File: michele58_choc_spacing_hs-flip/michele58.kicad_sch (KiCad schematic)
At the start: 103 parts, among them J1 OLED, J2 i2c, J3 i2c, J4 LED, U1 EliteC_Pro_Micro, U2 TRRS

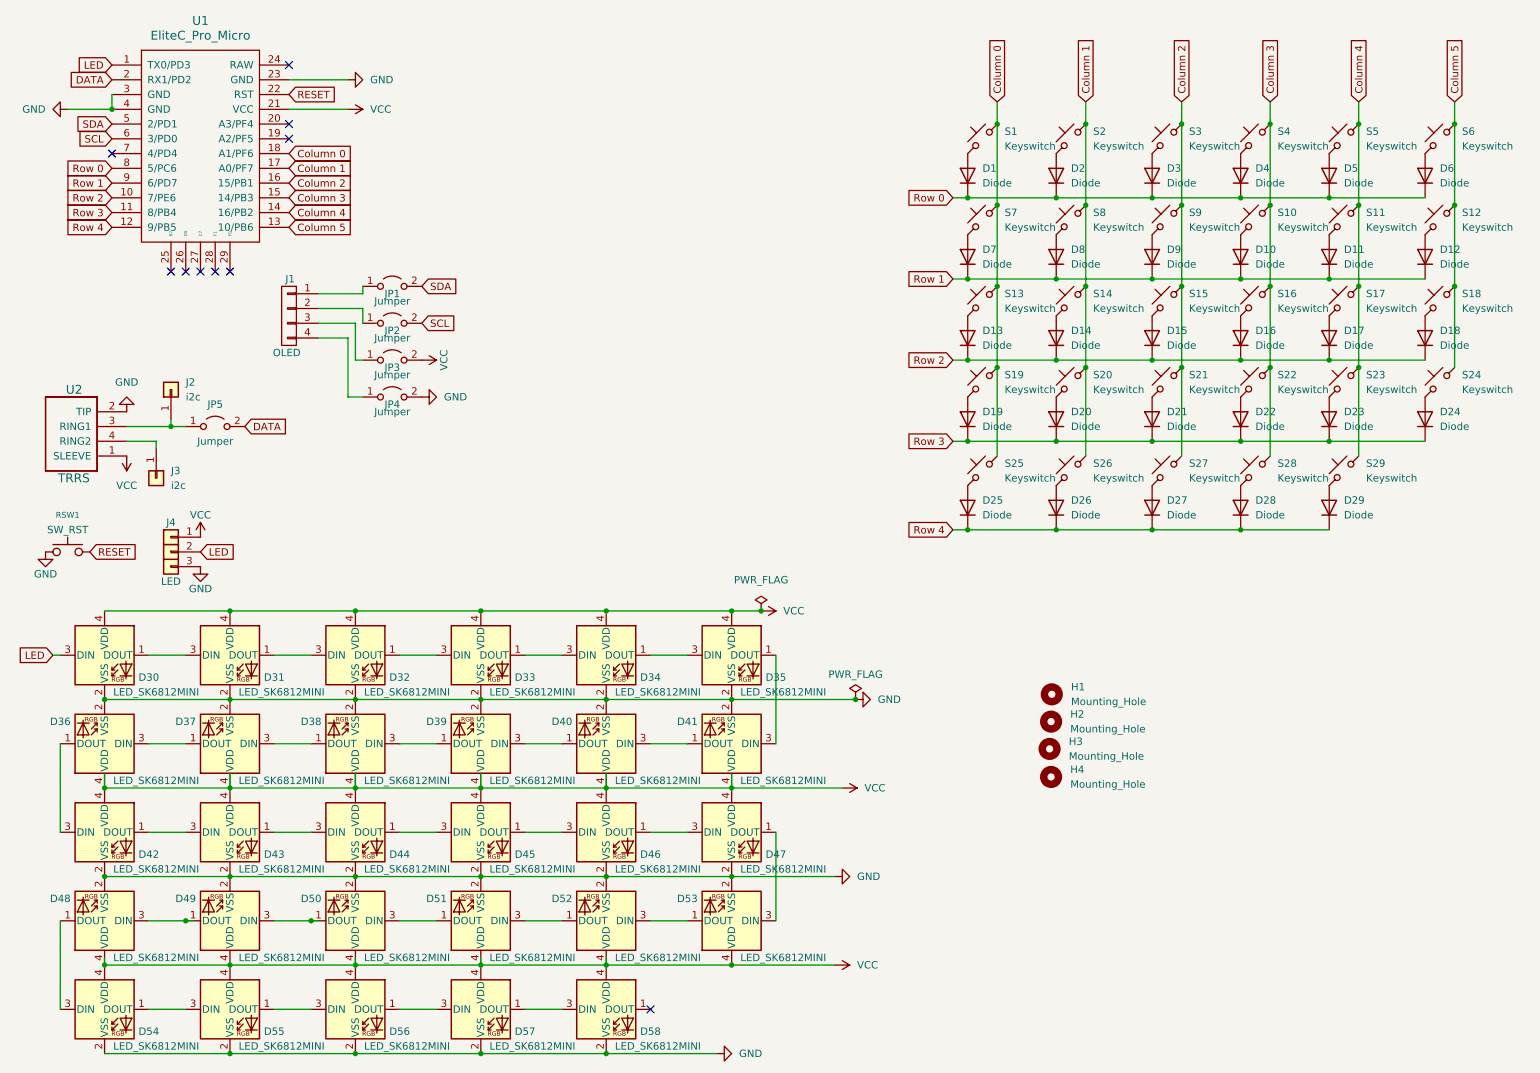
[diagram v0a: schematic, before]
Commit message: latest changes
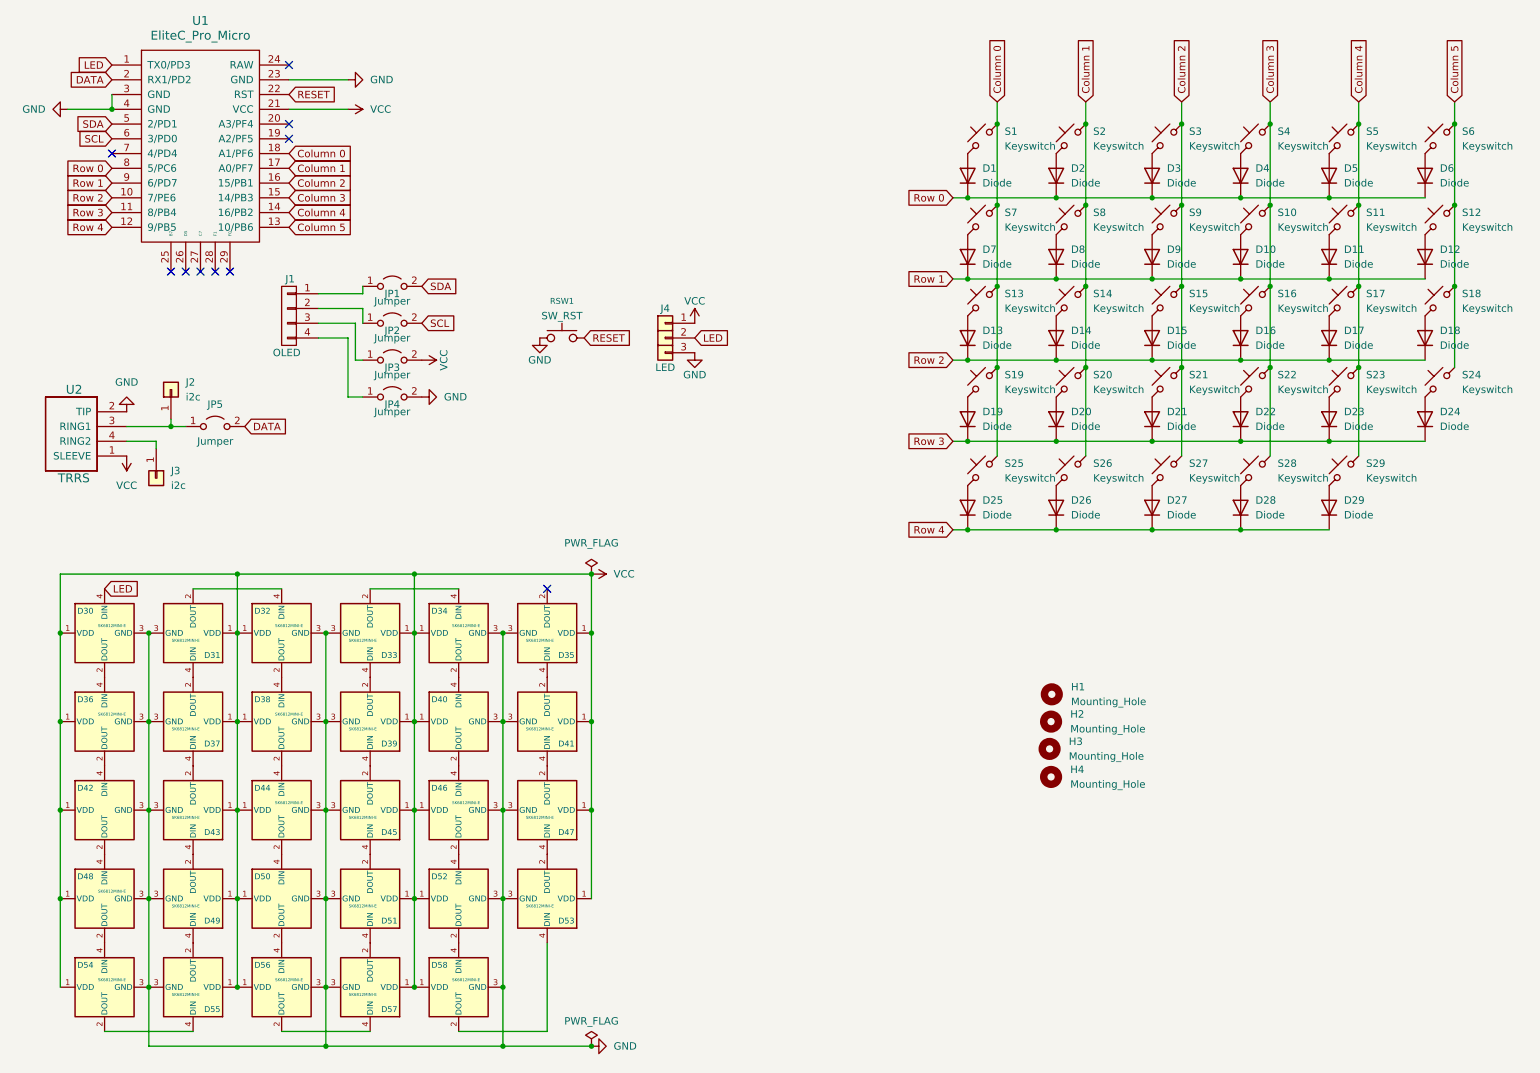
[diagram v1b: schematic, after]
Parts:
- D30: value LED_SK6812MINI -> SK6812MINI-E; symbol ScottoKeebs:LED_SK6812MINI -> SofleKeyboard1:LED_SK6812MINI-E-alt
- D31: renamed from D36; value LED_SK6812MINI -> SK6812MINI-E; symbol ScottoKeebs:LED_SK6812MINI -> SofleKeyboard1:LED_SK6812MINI-E-alt
- D32: renamed from D42; value LED_SK6812MINI -> SK6812MINI-E; symbol ScottoKeebs:LED_SK6812MINI -> SofleKeyboard1:LED_SK6812MINI-E-alt
- D33: renamed from D48; value LED_SK6812MINI -> SK6812MINI-E; symbol ScottoKeebs:LED_SK6812MINI -> SofleKeyboard1:LED_SK6812MINI-E-alt
- D34: renamed from D54; value LED_SK6812MINI -> SK6812MINI-E; symbol ScottoKeebs:LED_SK6812MINI -> SofleKeyboard1:LED_SK6812MINI-E-alt
- D35: renamed from D31; value LED_SK6812MINI -> SK6812MINI-E; symbol ScottoKeebs:LED_SK6812MINI -> SofleKeyboard1:LED_SK6812MINI-E-alt
- D36: renamed from D37; value LED_SK6812MINI -> SK6812MINI-E; symbol ScottoKeebs:LED_SK6812MINI -> SofleKeyboard1:LED_SK6812MINI-E-alt
- D37: renamed from D43; value LED_SK6812MINI -> SK6812MINI-E; symbol ScottoKeebs:LED_SK6812MINI -> SofleKeyboard1:LED_SK6812MINI-E-alt
- D38: renamed from D49; value LED_SK6812MINI -> SK6812MINI-E; symbol ScottoKeebs:LED_SK6812MINI -> SofleKeyboard1:LED_SK6812MINI-E-alt
- D39: renamed from D55; value LED_SK6812MINI -> SK6812MINI-E; symbol ScottoKeebs:LED_SK6812MINI -> SofleKeyboard1:LED_SK6812MINI-E-alt
- D40: renamed from D32; value LED_SK6812MINI -> SK6812MINI-E; symbol ScottoKeebs:LED_SK6812MINI -> SofleKeyboard1:LED_SK6812MINI-E-alt
- D41: renamed from D38; value LED_SK6812MINI -> SK6812MINI-E; symbol ScottoKeebs:LED_SK6812MINI -> SofleKeyboard1:LED_SK6812MINI-E-alt
- D42: renamed from D44; value LED_SK6812MINI -> SK6812MINI-E; symbol ScottoKeebs:LED_SK6812MINI -> SofleKeyboard1:LED_SK6812MINI-E-alt
- D43: renamed from D50; value LED_SK6812MINI -> SK6812MINI-E; symbol ScottoKeebs:LED_SK6812MINI -> SofleKeyboard1:LED_SK6812MINI-E-alt
- D44: renamed from D56; value LED_SK6812MINI -> SK6812MINI-E; symbol ScottoKeebs:LED_SK6812MINI -> SofleKeyboard1:LED_SK6812MINI-E-alt
- D45: renamed from D33; value LED_SK6812MINI -> SK6812MINI-E; symbol ScottoKeebs:LED_SK6812MINI -> SofleKeyboard1:LED_SK6812MINI-E-alt
- D46: renamed from D39; value LED_SK6812MINI -> SK6812MINI-E; symbol ScottoKeebs:LED_SK6812MINI -> SofleKeyboard1:LED_SK6812MINI-E-alt
- D47: renamed from D45; value LED_SK6812MINI -> SK6812MINI-E; symbol ScottoKeebs:LED_SK6812MINI -> SofleKeyboard1:LED_SK6812MINI-E-alt
- D48: renamed from D51; value LED_SK6812MINI -> SK6812MINI-E; symbol ScottoKeebs:LED_SK6812MINI -> SofleKeyboard1:LED_SK6812MINI-E-alt
- D49: renamed from D57; value LED_SK6812MINI -> SK6812MINI-E; symbol ScottoKeebs:LED_SK6812MINI -> SofleKeyboard1:LED_SK6812MINI-E-alt
- D50: renamed from D34; value LED_SK6812MINI -> SK6812MINI-E; symbol ScottoKeebs:LED_SK6812MINI -> SofleKeyboard1:LED_SK6812MINI-E-alt
- D51: renamed from D40; value LED_SK6812MINI -> SK6812MINI-E; symbol ScottoKeebs:LED_SK6812MINI -> SofleKeyboard1:LED_SK6812MINI-E-alt
- D52: renamed from D46; value LED_SK6812MINI -> SK6812MINI-E; symbol ScottoKeebs:LED_SK6812MINI -> SofleKeyboard1:LED_SK6812MINI-E-alt
- D53: renamed from D52; value LED_SK6812MINI -> SK6812MINI-E; symbol ScottoKeebs:LED_SK6812MINI -> SofleKeyboard1:LED_SK6812MINI-E-alt
- D54: renamed from D58; value LED_SK6812MINI -> SK6812MINI-E; symbol ScottoKeebs:LED_SK6812MINI -> SofleKeyboard1:LED_SK6812MINI-E-alt
- D55: renamed from D35; value LED_SK6812MINI -> SK6812MINI-E; symbol ScottoKeebs:LED_SK6812MINI -> SofleKeyboard1:LED_SK6812MINI-E-alt
- D56: renamed from D41; value LED_SK6812MINI -> SK6812MINI-E; symbol ScottoKeebs:LED_SK6812MINI -> SofleKeyboard1:LED_SK6812MINI-E-alt
- D57: renamed from D47; value LED_SK6812MINI -> SK6812MINI-E; symbol ScottoKeebs:LED_SK6812MINI -> SofleKeyboard1:LED_SK6812MINI-E-alt
- D58: renamed from D53; value LED_SK6812MINI -> SK6812MINI-E; symbol ScottoKeebs:LED_SK6812MINI -> SofleKeyboard1:LED_SK6812MINI-E-alt
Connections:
- net GND: now also D30.3 (GND), D31.3 (GND), D32.3 (GND), D33.3 (GND), D34.3 (GND), D35.3 (GND), D36.3 (GND), D37.3 (GND), D38.3 (GND), D39.3 (GND), D40.3 (GND), D41.3 (GND), D42.3 (GND), D43.3 (GND), D44.3 (GND), D45.3 (GND), D46.3 (GND), D47.3 (GND), D48.3 (GND), D49.3 (GND), D50.3 (GND), D51.3 (GND), D52.3 (GND), D53.3 (GND), D54.3 (GND), D55.3 (GND), D56.3 (GND), D57.3 (GND), D58.3 (GND); no longer D30.2 (VSS), D31.2 (VSS), D32.2 (VSS), D33.2 (VSS), D34.2 (VSS), D35.2 (VSS), D36.2 (VSS), D37.2 (VSS), D38.2 (VSS), D39.2 (VSS), D40.2 (VSS), D41.2 (VSS), D42.2 (VSS), D43.2 (VSS), D44.2 (VSS), D45.2 (VSS), D46.2 (VSS), D47.2 (VSS), D48.2 (VSS), D49.2 (VSS), D50.2 (VSS), D51.2 (VSS), D52.2 (VSS), D53.2 (VSS), D54.2 (VSS), D55.2 (VSS), D56.2 (VSS), D57.2 (VSS), D58.2 (VSS)
- net LED: now also D30.4 (DIN); no longer D30.3 (DIN)
- net VCC: now also D30.1 (VDD), D31.1 (VDD), D32.1 (VDD), D33.1 (VDD), D34.1 (VDD), D35.1 (VDD), D36.1 (VDD), D37.1 (VDD), D38.1 (VDD), D39.1 (VDD), D40.1 (VDD), D41.1 (VDD), D42.1 (VDD), D43.1 (VDD), D44.1 (VDD), D45.1 (VDD), D46.1 (VDD), D47.1 (VDD), D48.1 (VDD), D49.1 (VDD), D50.1 (VDD), D51.1 (VDD), D52.1 (VDD), D53.1 (VDD), D54.1 (VDD), D55.1 (VDD), D56.1 (VDD), D57.1 (VDD), D58.1 (VDD); no longer D30.4 (VDD), D31.4 (VDD), D32.4 (VDD), D33.4 (VDD), D34.4 (VDD), D35.4 (VDD), D36.4 (VDD), D37.4 (VDD), D38.4 (VDD), D39.4 (VDD), D40.4 (VDD), D41.4 (VDD), D42.4 (VDD), D43.4 (VDD), D44.4 (VDD), D45.4 (VDD), D46.4 (VDD), D47.4 (VDD), D48.4 (VDD), D49.4 (VDD), D50.4 (VDD), D51.4 (VDD), D52.4 (VDD), D53.4 (VDD), D54.4 (VDD), D55.4 (VDD), D56.4 (VDD), D57.4 (VDD), D58.4 (VDD)
- new net: D37.4 (DIN), D43.2 (DOUT)
- new net: D43.4 (DIN), D49.2 (DOUT)
- new net: D31.2 (DOUT), D32.4 (DIN)
- new net: D31.4 (DIN), D37.2 (DOUT)
- new net: D33.4 (DIN), D39.2 (DOUT)
- new net: D39.4 (DIN), D45.2 (DOUT)
- new net: D47.4 (DIN), D53.2 (DOUT)
- new net: D53.4 (DIN), D58.2 (DOUT)
- new net: D40.2 (DOUT), D46.4 (DIN)
- new net: D34.2 (DOUT), D40.4 (DIN)
- new net: D49.4 (DIN), D55.2 (DOUT)
- new net: D54.2 (DOUT), D55.4 (DIN)
- new net: D35.4 (DIN), D41.2 (DOUT)
- new net: D52.2 (DOUT), D58.4 (DIN)
- new net: D42.2 (DOUT), D48.4 (DIN)
- new net: D36.2 (DOUT), D42.4 (DIN)
- new net: D44.2 (DOUT), D50.4 (DIN)
- new net: D38.2 (DOUT), D44.4 (DIN)
- new net: D45.4 (DIN), D51.2 (DOUT)
- new net: D51.4 (DIN), D57.2 (DOUT)
- new net: D46.2 (DOUT), D52.4 (DIN)
- new net: D32.2 (DOUT), D38.4 (DIN)
- new net: D56.2 (DOUT), D57.4 (DIN)
- new net: D50.2 (DOUT), D56.4 (DIN)
- new net: D30.2 (DOUT), D36.4 (DIN)
- new net: D41.4 (DIN), D47.2 (DOUT)
- new net: D33.2 (DOUT), D34.4 (DIN)
- new net: D48.2 (DOUT), D54.4 (DIN)
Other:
- moved on the sheet: J4, RSW1
